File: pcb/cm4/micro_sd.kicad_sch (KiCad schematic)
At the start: 5 parts, among them J401 Micro_SD_Card, U401 RT9742GGJ5

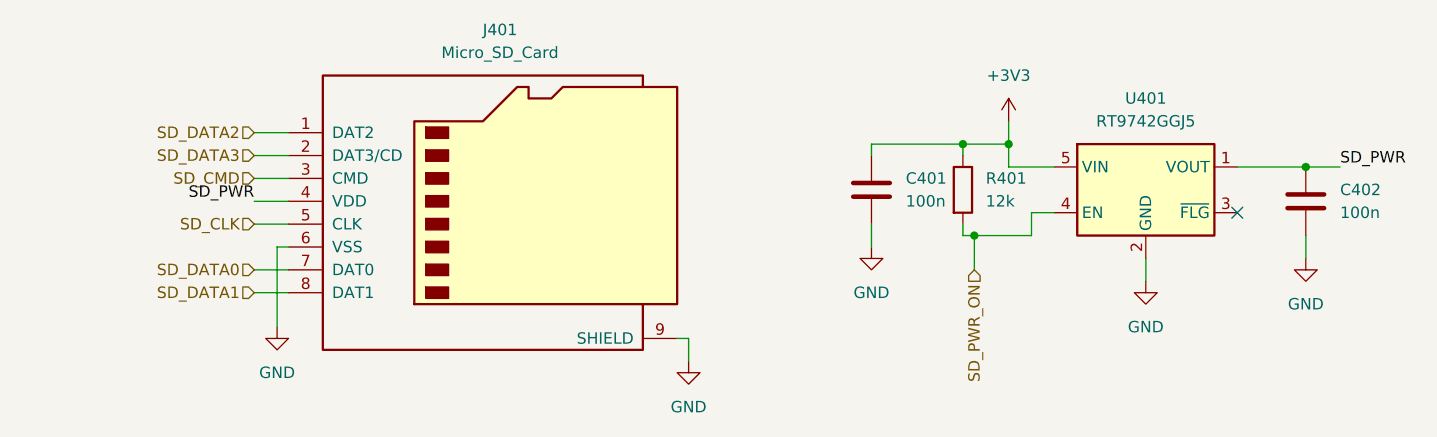
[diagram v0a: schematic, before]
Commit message: update cm4 board
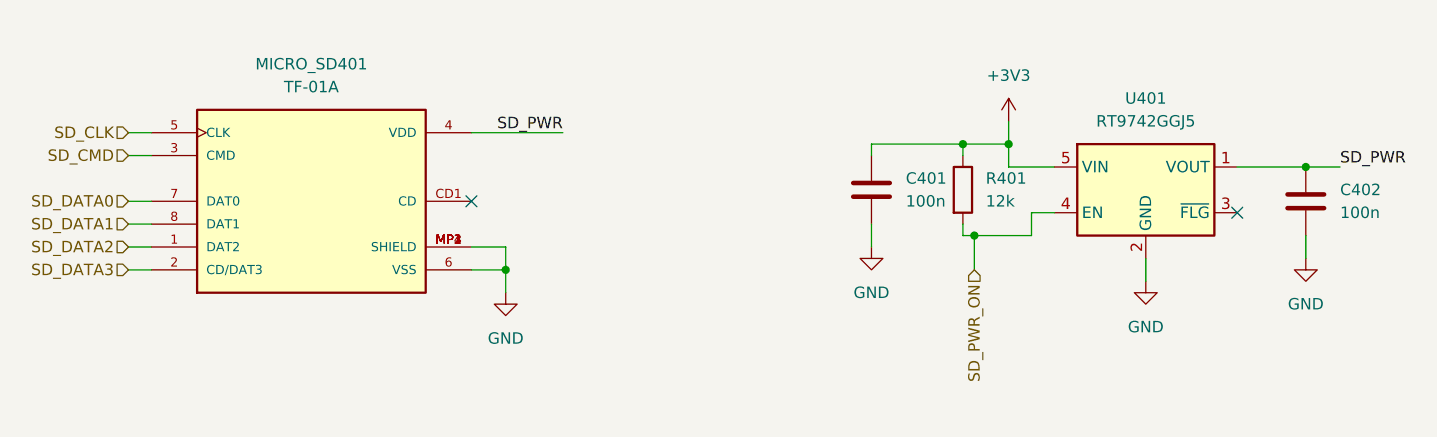
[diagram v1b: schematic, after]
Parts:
- removed J401: Micro_SD_Card, Connector_Card:microSD_HC_Wuerth_693072010801, symbol Connector:Micro_SD_Card
- added MICRO_SD401: TF-01A, DF40C-100DS-0.4V_51_:TF-01A, symbol TF-01A:TF-01A
- U401: LCSC (none) -> C250547
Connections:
- net GND: now also MICRO_SD401.6 (VSS), MICRO_SD401.MP1 (SHIELD), MICRO_SD401.MP2 (SHIELD), MICRO_SD401.MP3 (SHIELD), MICRO_SD401.MP4 (SHIELD)
- net SD_CLK: now also MICRO_SD401.5 (CLK)
- net SD_CMD: now also MICRO_SD401.3 (CMD)
- net SD_DATA0: now also MICRO_SD401.7 (DAT0)
- net SD_DATA1: now also MICRO_SD401.8 (DAT1)
- net SD_DATA2: now also MICRO_SD401.1 (DAT2)
- net SD_DATA3: now also MICRO_SD401.2 (CD/DAT3)
- net SD_PWR: now also MICRO_SD401.4 (VDD)
- no-connect marks 1 -> 2
